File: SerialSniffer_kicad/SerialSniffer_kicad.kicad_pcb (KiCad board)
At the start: 2 copper layers, 92.9 x 32 mm, 24 parts, among them J1 DE9_Plug_MountingHoles, J2 DE9_Receptacle_MountingHoles, J3 Conn_01x10, J4 Conn_01x02, J5 Conn_02x02_Odd_Even, J6 Conn_02x02_Odd_Even, J7 STM32F401, J8 Conn_02x02_Odd_Even, U1 74HC14

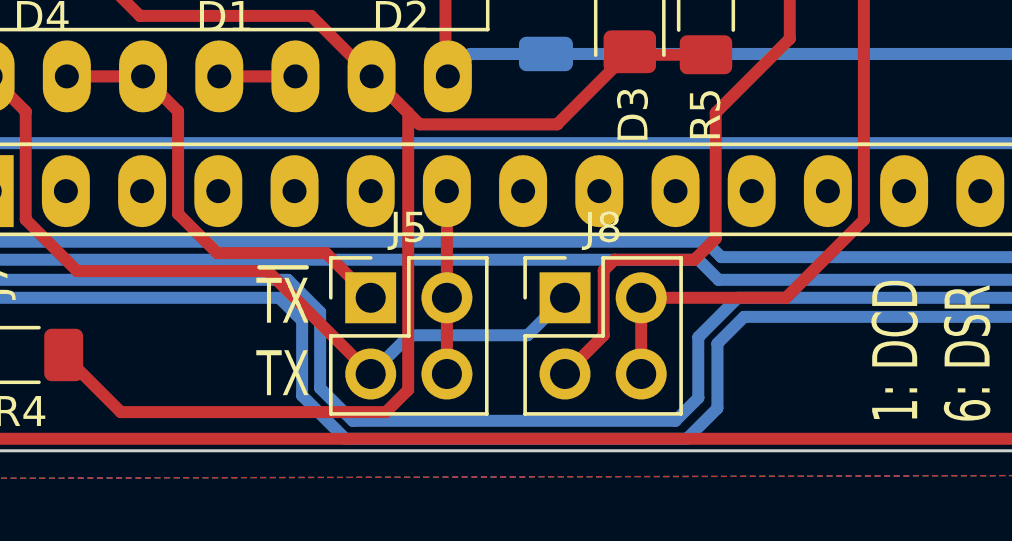
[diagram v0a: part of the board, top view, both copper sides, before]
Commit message: Initial
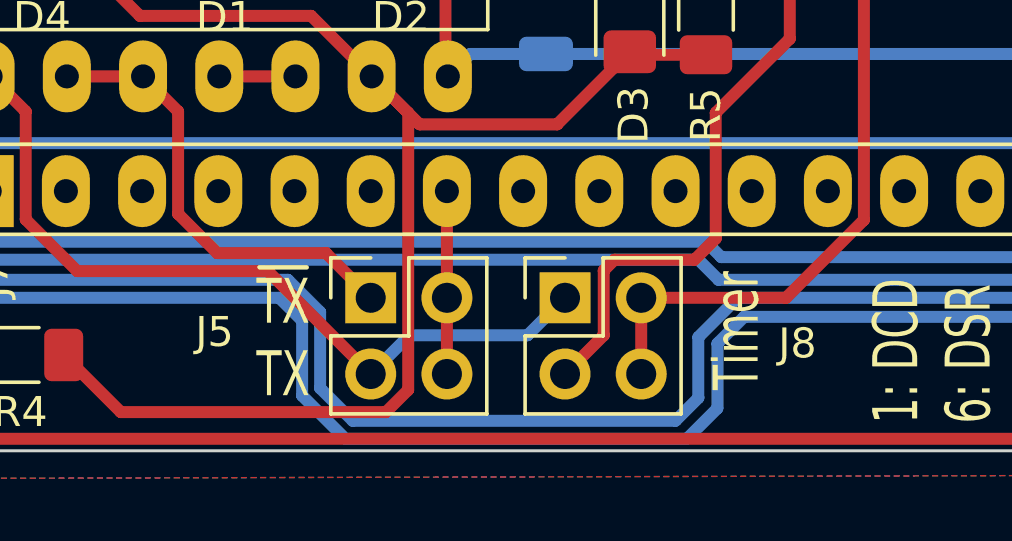
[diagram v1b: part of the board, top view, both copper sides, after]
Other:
- board text added: "Timer"
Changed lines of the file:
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@@
 		(tags "Through hole pin header THT 2x02 2.54mm double row")
 		(property "Reference" "J5"
-			(at 1.27 -2.33 0)
+			(at -5.207 1.143 0)
 			(layer "F.SilkS")
 			(effects
@@
 			(at 1.27 4.87 0)
 			(layer "F.Fab")
+			(hide yes)
 			(effects
 				(font
@@
 		(tags "Through hole pin header THT 2x02 2.54mm double row")
 		(property "Reference" "J8"
-			(at 1.27 -2.33 0)
+			(at 7.747 1.524 0)
 			(layer "F.SilkS")
 			(effects
@@
 			(at 1.27 4.87 0)
 			(layer "F.Fab")
+			(hide yes)
 			(effects
 				(font
@@
 		(layer "Edge.Cuts")
 	)
+	(gr_text "Timer"
+		(at 119.761 96.012 90)
+		(layer "F.SilkS")
+		(effects
+			(font
+				(face "DejaVu Sans Mono")
+				(size 1.5 1)
+				(thickness 0.15)
+			)
+			(justify right bottom)
+		)
+		(render_cache "Timer" 90
+			(polygon
+				(pts
+					(xy 117.958477 100.190505) (xy 117.958477 99.407951) (xy 118.122608 99.407951) (xy 118.122608 99.728886)
+					(xy 119.506 99.728886) (xy 119.506 99.868349) (xy 118.122608 99.868349) (xy 118.122608 100.190505)
+				)
+			)
+			(polygon
+				(pts
+					(xy 118.357081 99.204741) (xy 118.357081 98.88112) (xy 119.365316 98.88112) (xy 119.365316 98.630526)
+					(xy 119.506 98.630526) (xy 119.506 99.25823) (xy 119.365316 99.25823) (xy 119.365316 99.007637)
+					(xy 118.497765 99.007637) (xy 118.497765 99.204741)
+				)
+			)
+			(polygon
+				(pts
+					(xy 117.911582 99.007637) (xy 117.911582 98.88112) (xy 118.146055 98.88112) (xy 118.146055 99.007637)
+				)
+			)
+			(polygon
+				(pts
+					(xy 118.483477 98.074141) (xy 118.41689 98.04758) (xy 118.37027 98.01479) (xy 118.340646 97.969487)
+					(xy 118.333634 97.92784) (xy 118.344152 97.875175) (xy 118.380021 97.829585) (xy 118.441345 97.796926)
+					(xy 118.516973 97.778507) (xy 118.596592 97.768349) (xy 118.67932 97.762545) (xy 118.758473 97.759754)
+					(xy 118.84691 97.758824) (xy 119.506 97.758824) (xy 119.506 97.874106) (xy 118.855337 97.874106)
+					(xy 118.771488 97.87475) (xy 118.689878 97.87713) (xy 118.610608 97.882764) (xy 118.556383 97.892424)
+					(xy 118.504692 97.929085) (xy 118.497765 97.958614) (xy 118.515446 98.007215) (xy 118.560413 98.033841)
+					(xy 118.639133 98.046967) (xy 118.715526 98.051718) (xy 118.799838 98.053797) (xy 118.855337 98.054113)
+					(xy 119.506 98.054113) (xy 119.506 98.16964) (xy 118.855337 98.16964) (xy 118.770543 98.170327)
+					(xy 118.688222 98.172865) (xy 118.608656 98.178876) (xy 118.554918 98.18918) (xy 118.505802 98.225816)
+					(xy 118.497765 98.259521) (xy 118.519851 98.30842) (xy 118.560413 98.329375) (xy 118.639133 98.342026)
+					(xy 118.715526 98.346606) (xy 118.799838 98.348609) (xy 118.855337 98.348914) (xy 119.506 98.348914)
+					(xy 119.506 98.463464) (xy 118.357081 98.463464) (xy 118.357081 98.348914) (xy 118.463327 98.348914)
+					(xy 118.401644 98.319806) (xy 118.366973 98.29225) (xy 118.338322 98.246187) (xy 118.333634 98.215069)
+					(xy 118.34418 98.164498) (xy 118.371003 98.128119) (xy 118.424803 98.09397)
+				)
+			)
+			(polygon
+				(pts
+					(xy 118.990159 97.479898) (xy 118.995654 97.479898) (xy 119.069089 97.476766) (xy 119.143656 97.465516)
+					(xy 119.21561 97.443079) (xy 119.268962 97.414441) (xy 119.315539 97.373215) (xy 119.346873 97.323448)
+					(xy 119.361928 97.272043) (xy 119.365316 97.229061) (xy 119.360539 97.179117) (xy 119.346209 97.127319)
+					(xy 119.336373 97.102787) (xy 119.312716 97.056382) (xy 119.282046 97.007841) (xy 119.248079 96.961859)
+					(xy 119.435658 96.961859) (xy 119.465127 97.010818) (xy 119.489055 97.058621) (xy 119.506 97.101078)
+					(xy 119.520288 97.150651) (xy 119.528325 97.202961) (xy 119.529447 97.230526) (xy 119.525565 97.284641)
+					(xy 119.513919 97.33494) (xy 119.489696 97.390261) (xy 119.454293 97.440087) (xy 119.407711 97.484417)
+					(xy 119.370445 97.510917) (xy 119.306457 97.545198) (xy 119.23402 97.572386) (xy 119.153133 97.592482)
+					(xy 119.079274 97.60381) (xy 118.999547 97.610213) (xy 118.93154 97.611789) (xy 118.849044 97.609374)
+					(xy 118.771914 97.602129) (xy 118.700151 97.590054) (xy 118.62112 97.569189) (xy 118.549816 97.541368)
+					(xy 118.4963 97.512871) (xy 118.441019 97.473458) (xy 118.397175 97.429409) (xy 118.364769 97.380722)
+					(xy 118.3438 97.327399) (xy 118.334269 97.269439) (xy 118.333802 97.254462) (xy 118.497765 97.254462)
+					(xy 118.505155 97.303295) (xy 118.5307 97.351571) (xy 118.574492 97.39355) (xy 118.591188 97.404916)
+					(xy 118.656661 97.437159) (xy 118.727701 97.458142) (xy 118.800481 97.470404) (xy 118.850574 97.475013)
+					(xy 118.849475 97.058824) (xy 118.768531 97.063113) (xy 118.689786 97.074982) (xy 118.617587 97.096916)
+					(xy 118.587524 97.111336) (xy 118.536421 97.150728) (xy 118.506531 97.200395) (xy 118.497765 97.254462)
+					(xy 118.333802 97.254462) (xy 118.333634 97.249089) (xy 118.338992 97.196141) (xy 118.355066 97.147572)
+					(xy 118.387363 97.096443) (xy 118.434247 97.051274) (xy 118.486041 97.017302) (xy 118.54711 96.988417)
+					(xy 118.616009 96.965508) (xy 118.69274 96.948575) (xy 118.777301 96.937618) (xy 118.853751 96.933053)
+					(xy 118.902231 96.932306) (xy 118.990159 96.932306)
+				)
+			)
+			(polygon
+				(pts
+					(xy 118.591554 96.060847) (xy 118.549148 96.101758) (xy 118.520113 96.143401) (xy 118.502043 96.193015)
+					(xy 118.497765 96.235237) (xy 118.50313 96.28429) (xy 118.522398 96.333826) (xy 118.560825 96.381233)
+					(xy 118.609872 96.415976) (xy 118.671971 96.443332) (xy 118.746526 96.462871) (xy 118.82198 96.473557)
+					(xy 118.906971 96.478258) (xy 118.933006 96.478503) (xy 119.506 96.478503) (xy 119.506 96.605509)
+					(xy 118.357081 96.605509) (xy 118.357081 96.478503) (xy 118.578732 96.478503) (xy 118.509981 96.455471)
+					(xy 118.446918 96.422423) (xy 118.397015 96.381294) (xy 118.36093 96.333267) (xy 118.341123 96.284648)
+					(xy 118.333696 96.231305) (xy 118.333634 96.225711) (xy 118.339082 96.175162) (xy 118.350853 96.138517)
+					(xy 118.377711 96.091576) (xy 118.403976 96.060847)
+				)
+			)
+		)
+	)
 	(gr_text "RX\n~{RX}\n"
